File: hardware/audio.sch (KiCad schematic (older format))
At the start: 10 parts, among them J2 Conn_01x02, J3 Conn_01x02, U3 SPH0645LM4H-B, U5 MAX98357AETE+T

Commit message: update
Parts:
- removed J2, J3: Conn_01x02, Connector_PinHeader_1.00mm:PinHeader_1x02_P1.00mm_Vertical, symbol Connector_Generic:Conn_01x02
- C5, C6: footprint Capacitor_SMD:C_0603_1608Metric_Pad0.99x1.00mm_HandSolder -> Capacitor_SMD:C_0603_1608Metric_Pad1.05x0.95mm_HandSolder
- R11, R17, R9: footprint Resistors_SMD:R_0603_HandSoldering -> Resistor_SMD:R_0603_1608Metric_Pad1.05x0.95mm_HandSolder
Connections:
- wire segments 41 -> 39
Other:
- moved on the sheet: LS1
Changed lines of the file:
@@
 F 0 "R11" V 4750 4150 50  0000 C CNN
 F 1 "R_47.5" V 4675 4150 50  0000 C CNN
-F 2 "Resistors_SMD:R_0603_HandSoldering" V 4680 4150 50  0001 C CNN
+F 2 "Resistor_SMD:R_0603_1608Metric_Pad1.05x0.95mm_HandSolder" V 4680 4150 50  0001 C CNN
 F 3 "https://www.digikey.com/product-detail/en/yageo/RC0603FR-0747R5L/311-47.5HRCT-ND/730201" V 4830 4150 50  0001 C CNN
 F 4 "RC0603FR-0747R5L" V 4930 4250 60  0001 C CNN "Part Number"
@@
 F 0 "R9" V 4750 3950 50  0000 C CNN
 F 1 "R_100k" V 4650 3950 50  0000 C CNN
-F 2 "Resistors_SMD:R_0603_HandSoldering" V 4680 3950 50  0001 C CNN
+F 2 "Resistor_SMD:R_0603_1608Metric_Pad1.05x0.95mm_HandSolder" V 4680 3950 50  0001 C CNN
 F 3 "https://www.digikey.com/product-detail/en/yageo/RC0603JR-07100KL/311-100KGRCT-ND/729645" V 4830 3950 50  0001 C CNN
 F 4 "RC0603JR-07100KL" V 4930 4050 60  0001 C CNN "Part Number"
@@
 F 0 "R17" V 7000 4325 50  0000 C CNN
 F 1 "R_100k" V 6925 4325 50  0000 C CNN
-F 2 "Resistors_SMD:R_0603_HandSoldering" V 6930 4325 50  0001 C CNN
+F 2 "Resistor_SMD:R_0603_1608Metric_Pad1.05x0.95mm_HandSolder" V 6930 4325 50  0001 C CNN
 F 3 "https://www.digikey.com/product-detail/en/yageo/RC0603JR-07100KL/311-100KGRCT-ND/729645" V 7080 4325 50  0001 C CNN
 F 4 "RC0603JR-07100KL" V 7180 4425 60  0001 C CNN "Part Number"
@@
 L liger-rescue:speaker-CVS-1508 LS1
 U 1 1 5A1620B5
-P 9525 3950
-F 0 "LS1" H 9525 4075 50  0000 R CNN
-F 1 "speaker-CVS-1508" H 9575 4100 50  0001 R CNN
-F 2 "open-automation:speaker-1508" H 9525 3750 50  0001 C CNN
-F 3 "http://www.cui.com/product/resource/cvs-1508.pdf" H 9515 3900 50  0001 C CNN
-F 4 "CVS-1508" H 9675 4275 60  0001 C CNN "Part Number"
-	1    9525 3950
+P 8900 3950
+F 0 "LS1" H 8900 4075 50  0000 R CNN
+F 1 "speaker-CVS-1508" H 8950 4100 50  0001 R CNN
+F 2 "open-automation:speaker-1508" H 8900 3750 50  0001 C CNN
+F 3 "http://www.cui.com/product/resource/cvs-1508.pdf" H 8890 3900 50  0001 C CNN
+F 4 "CVS-1508" H 9050 4275 60  0001 C CNN "Part Number"
+	1    8900 3950
 	1    0    0    -1
 $EndComp
@@
 	8500 4150 8500 3950
 Wire Wire Line
-	8500 3950 8625 3950
-Wire Wire Line
 	8575 4250 8575 4050
-Wire Wire Line
-	8575 4050 8625 4050
 Text Label 7225 3525 0    197  ~ 0
 Speaker
@@
 F 0 "C5" H 3515 4596 50  0000 L CNN
 F 1 "C_0.1uF" H 3515 4505 50  0000 L CNN
-F 2 "Capacitor_SMD:C_0603_1608Metric_Pad0.99x1.00mm_HandSolder" H 3500 4850 50  0001 C CNN
+F 2 "Capacitor_SMD:C_0603_1608Metric_Pad1.05x0.95mm_HandSolder" H 3500 4850 50  0001 C CNN
 F 3 "https://www.digikey.com/product-detail/en/tdk-corporation/C1608X8R1H104K080AB/445-8818-1-ND/3248223" H 3400 4300 50  0001 C CNN
 F 4 "C1608X8R1H104K080AB" H 3525 4750 60  0001 C CNN "Part Number"
@@
 F 0 "C6" H 7115 4671 50  0000 L CNN
 F 1 "C_0.1uF" H 7115 4580 50  0000 L CNN
-F 2 "Capacitor_SMD:C_0603_1608Metric_Pad0.99x1.00mm_HandSolder" H 7100 4925 50  0001 C CNN
+F 2 "Capacitor_SMD:C_0603_1608Metric_Pad1.05x0.95mm_HandSolder" H 7100 4925 50  0001 C CNN
 F 3 "https://www.digikey.com/product-detail/en/tdk-corporation/C1608X8R1H104K080AB/445-8818-1-ND/3248223" H 7000 4375 50  0001 C CNN
 F 4 "C1608X8R1H104K080AB" H 7125 4825 60  0001 C CNN "Part Number"
@@
 3V3
 Wire Wire Line
-	9325 3950 9250 3950
-$Comp
-L Connector_Generic:Conn_01x02 J2
-U 1 1 5B2BE39C
-P 8825 3950
-F 0 "J2" H 8775 4050 50  0000 L CNN
-F 1 "Conn_01x02" H 8700 3725 50  0000 L CNN
-F 2 "Connector_PinHeader_1.00mm:PinHeader_1x02_P1.00mm_Vertical" H 8825 3950 50  0001 C CNN
-F 3 "~" H 8825 3950 50  0001 C CNN
-	1    8825 3950
-	1    0    0    -1
-$EndComp
-$Comp
-L Connector_Generic:Conn_01x02 J3
-U 1 1 5B2BE409
-P 9050 4050
-F 0 "J3" H 8970 3725 50  0000 C CNN
-F 1 "Conn_01x02" H 8970 3816 50  0000 C CNN
-F 2 "Connector_PinHeader_1.00mm:PinHeader_1x02_P1.00mm_Vertical" H 9050 4050 50  0001 C CNN
-F 3 "~" H 9050 4050 50  0001 C CNN
-	1    9050 4050
-	-1   0    0    1
-$EndComp
-Wire Wire Line
-	9250 4050 9325 4050
+	8500 3950 8700 3950
+Wire Wire Line
+	8575 4050 8700 4050
 $EndSCHEMATC

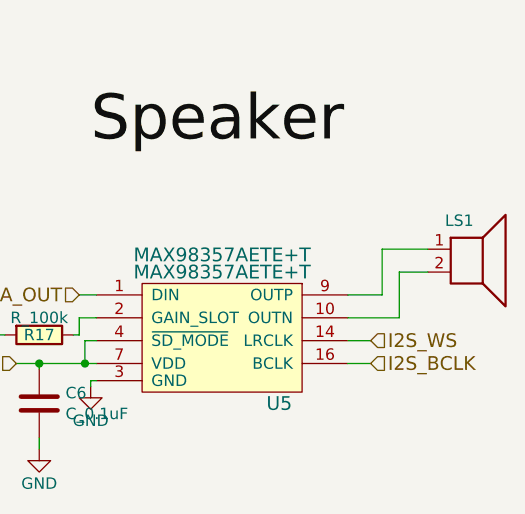
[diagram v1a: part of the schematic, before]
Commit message: update
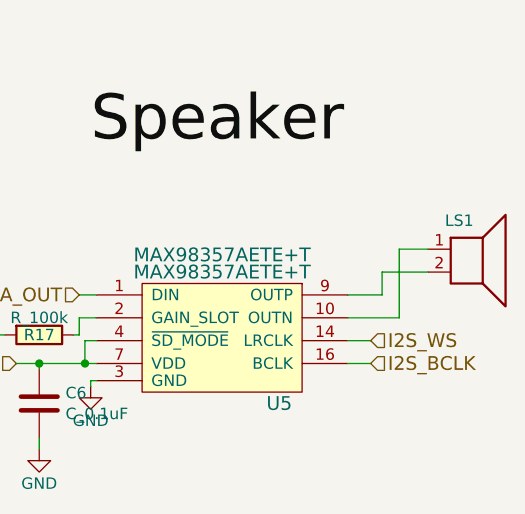
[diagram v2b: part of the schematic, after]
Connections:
- net at U5.10 (OUTN): now also LS1.1; no longer LS1.2
- net at U5.9 (OUTP): now also LS1.2; no longer LS1.1
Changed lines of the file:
@@
 	1    0    0    -1
 $EndComp
-Wire Wire Line
-	8500 4150 8500 3950
-Wire Wire Line
-	8575 4250 8575 4050
 Text Label 7225 3525 0    197  ~ 0
 Speaker
@@
 3V3
 Wire Wire Line
-	8500 3950 8700 3950
+	8700 4050 8500 4050
 Wire Wire Line
-	8575 4050 8700 4050
+	8500 4050 8500 4150
+Wire Wire Line
+	8700 3950 8575 3950
+Wire Wire Line
+	8575 3950 8575 4250
 $EndSCHEMATC

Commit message: order complete
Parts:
- C5, C6: Part Number C1608X8R1H104K080AB -> CL10F104ZO8NNNC
- R11: Part Number RC0603FR-0747R5L -> ERJ-3EKF47R5V
- R17, R9: Part Number RC0603JR-07100KL -> ERA-3AEB104V
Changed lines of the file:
@@
 F 2 "Resistor_SMD:R_0603_1608Metric_Pad1.05x0.95mm_HandSolder" V 4680 4150 50  0001 C CNN
 F 3 "https://www.digikey.com/product-detail/en/yageo/RC0603FR-0747R5L/311-47.5HRCT-ND/730201" V 4830 4150 50  0001 C CNN
-F 4 "RC0603FR-0747R5L" V 4930 4250 60  0001 C CNN "Part Number"
+F 4 "ERJ-3EKF47R5V" V 4930 4250 60  0001 C CNN "Part Number"
 	1    4750 4150
 	0    1    1    0
@@
 F 2 "Resistor_SMD:R_0603_1608Metric_Pad1.05x0.95mm_HandSolder" V 4680 3950 50  0001 C CNN
 F 3 "https://www.digikey.com/product-detail/en/yageo/RC0603JR-07100KL/311-100KGRCT-ND/729645" V 4830 3950 50  0001 C CNN
-F 4 "RC0603JR-07100KL" V 4930 4050 60  0001 C CNN "Part Number"
+F 4 "ERA-3AEB104V" V 4930 4050 60  0001 C CNN "Part Number"
 	1    4750 3950
 	0    1    1    0
@@
 F 2 "Resistor_SMD:R_0603_1608Metric_Pad1.05x0.95mm_HandSolder" V 6930 4325 50  0001 C CNN
 F 3 "https://www.digikey.com/product-detail/en/yageo/RC0603JR-07100KL/311-100KGRCT-ND/729645" V 7080 4325 50  0001 C CNN
-F 4 "RC0603JR-07100KL" V 7180 4425 60  0001 C CNN "Part Number"
+F 4 "ERA-3AEB104V" V 7180 4425 60  0001 C CNN "Part Number"
 	1    7000 4325
 	0    1    1    0
@@
 F 2 "Capacitor_SMD:C_0603_1608Metric_Pad1.05x0.95mm_HandSolder" H 3500 4850 50  0001 C CNN
 F 3 "https://www.digikey.com/product-detail/en/tdk-corporation/C1608X8R1H104K080AB/445-8818-1-ND/3248223" H 3400 4300 50  0001 C CNN
-F 4 "C1608X8R1H104K080AB" H 3525 4750 60  0001 C CNN "Part Number"
+F 4 "CL10F104ZO8NNNC" H 3525 4750 60  0001 C CNN "Part Number"
 	1    3400 4550
 	1    0    0    -1
@@
 F 2 "Capacitor_SMD:C_0603_1608Metric_Pad1.05x0.95mm_HandSolder" H 7100 4925 50  0001 C CNN
 F 3 "https://www.digikey.com/product-detail/en/tdk-corporation/C1608X8R1H104K080AB/445-8818-1-ND/3248223" H 7000 4375 50  0001 C CNN
-F 4 "C1608X8R1H104K080AB" H 7125 4825 60  0001 C CNN "Part Number"
+F 4 "CL10F104ZO8NNNC" H 7125 4825 60  0001 C CNN "Part Number"
 	1    7000 4625
 	1    0    0    -1
